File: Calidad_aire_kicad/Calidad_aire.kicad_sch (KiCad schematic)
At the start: 10 parts, among them J1 Micro_SD_Card, U1 DOIT-ESP32-DEVKIT-V1

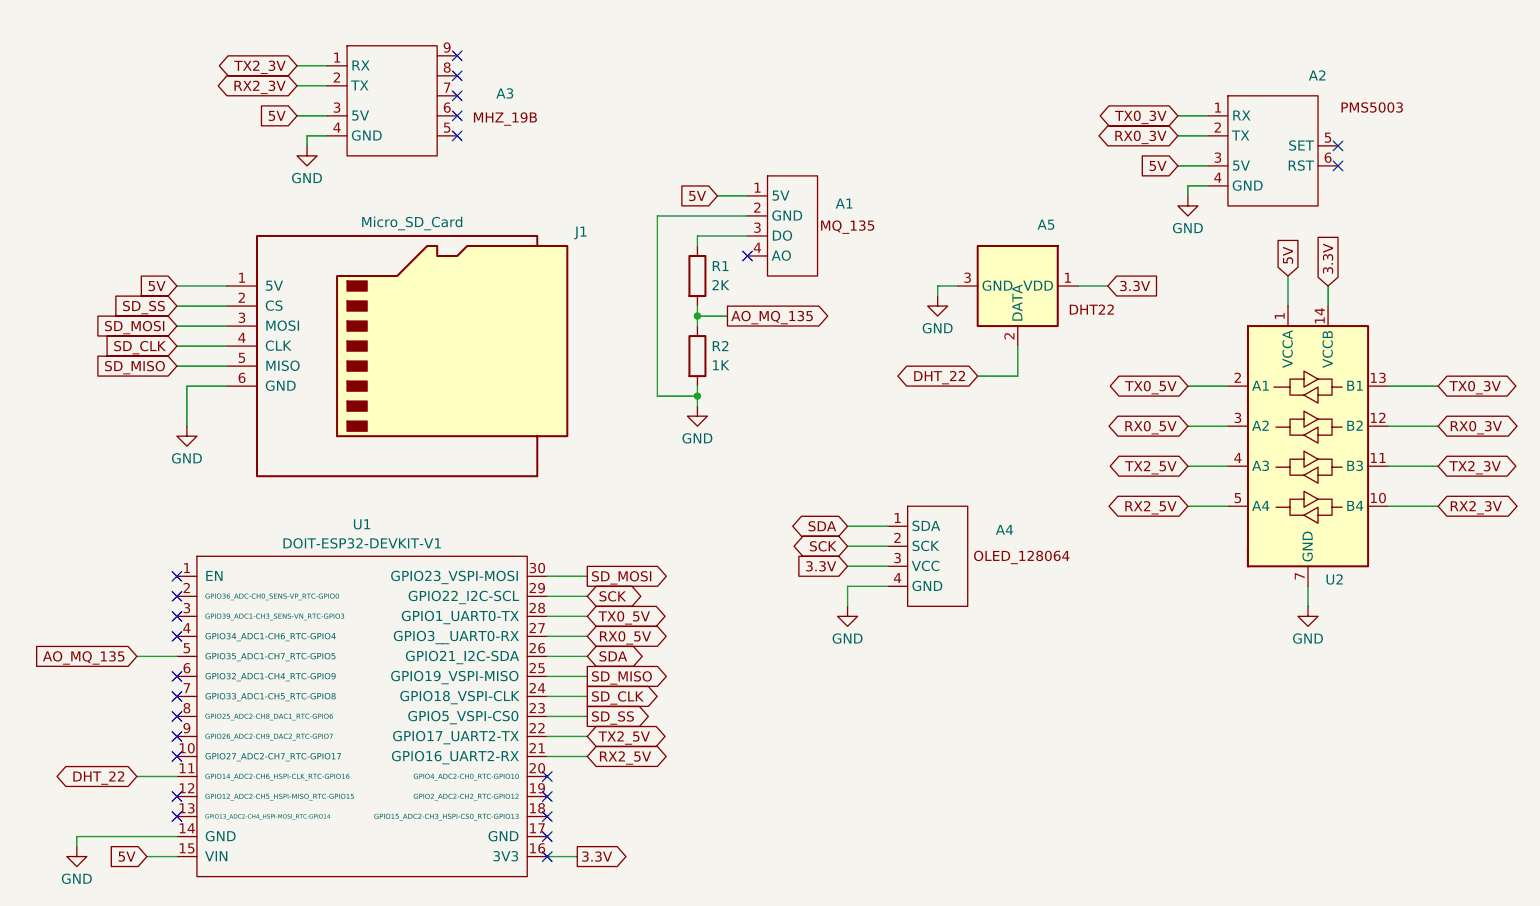
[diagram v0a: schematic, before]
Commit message: PCB design actualization
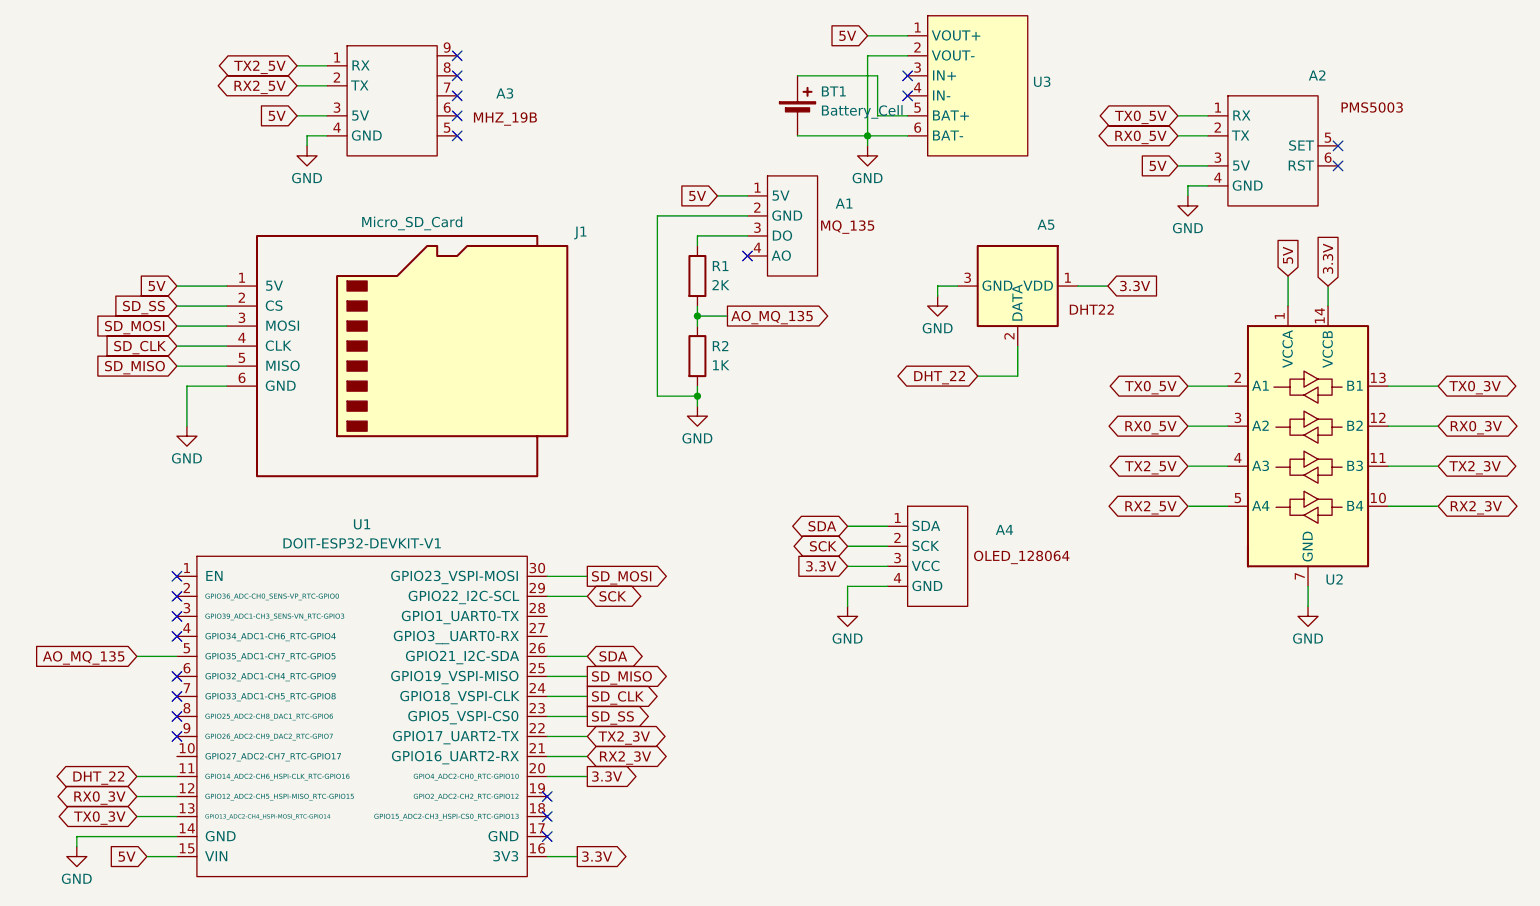
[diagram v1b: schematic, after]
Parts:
- added BT1: Battery_Cell, TerminalBlock:TerminalBlock_bornier-2_P5.08mm, symbol Device:Battery_Cell
- added U3: ~, footprint_project:USB_TP4056, symbol symbols:USB_TPC4056
- R1, R2: footprint (none) -> Resistor_THT:R_Axial_DIN0414_L11.9mm_D4.5mm_P15.24mm_Horizontal
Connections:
- net 3.3V: now also U1.20 (GPIO4_ADC2-CH0_RTC-GPIO10)
- net 5V: now also U3.1 (VOUT+)
- net GND: now also BT1.2 (-), U3.2 (VOUT-), U3.6 (BAT-)
- net RX0_3V: now also U1.12 (GPIO12_ADC2-CH5_HSPI-MISO_RTC-GPIO15); no longer A2.2 (TX)
- net RX0_5V: now also A2.2 (TX); no longer U1.27 (GPIO3__UART0-RX)
- net RX2_3V: now also U1.21 (GPIO16_UART2-RX); no longer A3.2 (TX)
- net RX2_5V: now also A3.2 (TX); no longer U1.21 (GPIO16_UART2-RX)
- net TX0_3V: now also U1.13 (GPIO13_ADC2-CH4_HSPI-MOSI_RTC-GPIO14); no longer A2.1 (RX)
- net TX0_5V: now also A2.1 (RX); no longer U1.28 (GPIO1_UART0-TX)
- net TX2_3V: now also U1.22 (GPIO17_UART2-TX); no longer A3.1 (RX)
- net TX2_5V: now also A3.1 (RX); no longer U1.22 (GPIO17_UART2-TX)
- new net: BT1.1 (+), U3.5 (BAT+)
- no-connect marks 24 -> 21
